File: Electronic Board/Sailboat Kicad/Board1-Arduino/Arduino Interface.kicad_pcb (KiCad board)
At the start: 2 copper layers, 70.5 x 101.6 mm, 54 parts, among them J1 Conn_01x02, J10 Conn_01x02, J11 Conn_01x03_Male, J12 Conn_01x03_Male, J13 Conn_01x03_Male, J14 Conn_01x03_Male, J15 Conn_01x04, J16 Conn_01x04, J17 Conn_01x04, J18 Conn_01x04, J19 Conn_01x03, J2 Conn_01x08, J20 Conn_01x03, J21 Conn_01x02, J22 Conn_01x02, J23 Conn_01x06, J24 Conn_01x03, J25 Conn_01x06, J26 Conn_02x02_Odd_Even, J3 Conn_01x08, J31 Conn_01x04, J32 Conn_01x04, J34 Conn_01x02, J35 Conn_01x02, J36 Conn_01x02, J37 Conn_01x02, J4 Conn_01x08, J5 Conn_02x18_Odd_Even, J6 Conn_01x08, J7 Conn_01x08, J8 Conn_01x08, J9 Conn_01x02, U1 L7805, U2 L7805, U3 L7805

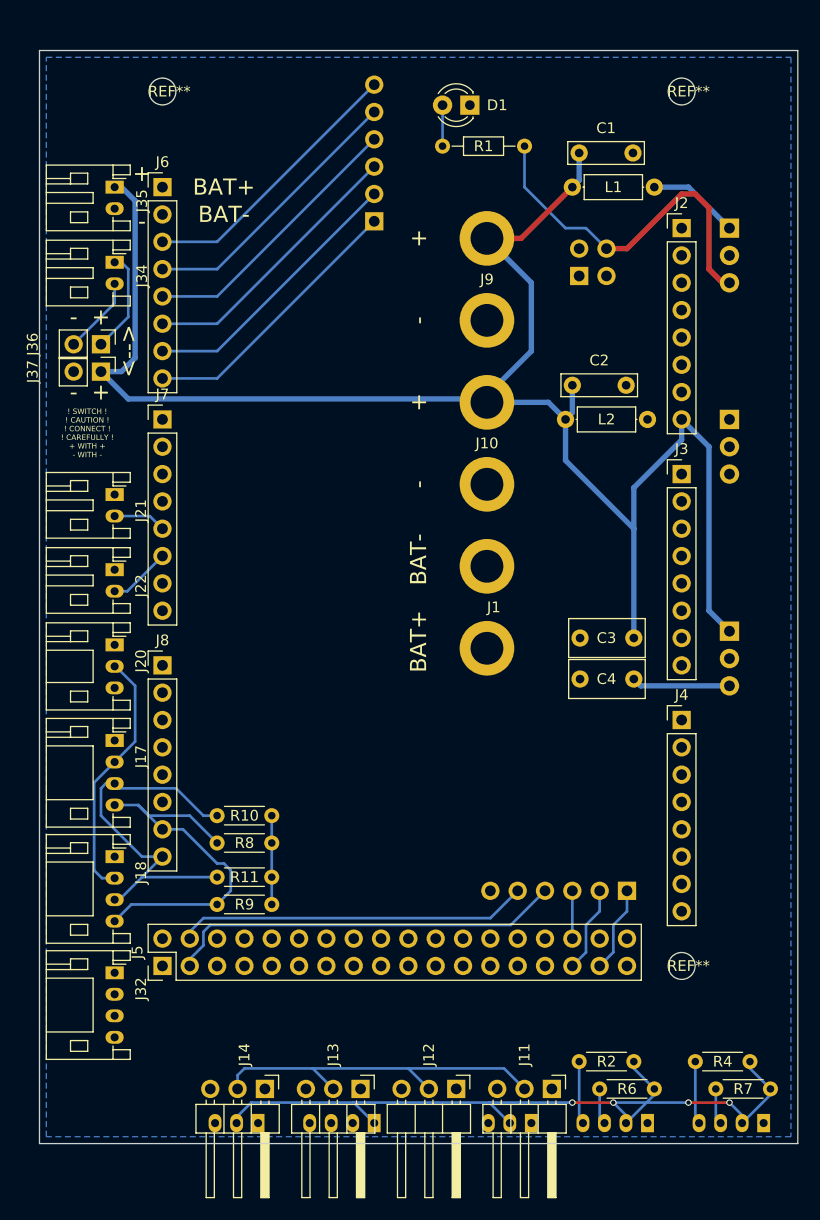
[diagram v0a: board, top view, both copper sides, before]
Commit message: Finished board-v0.1
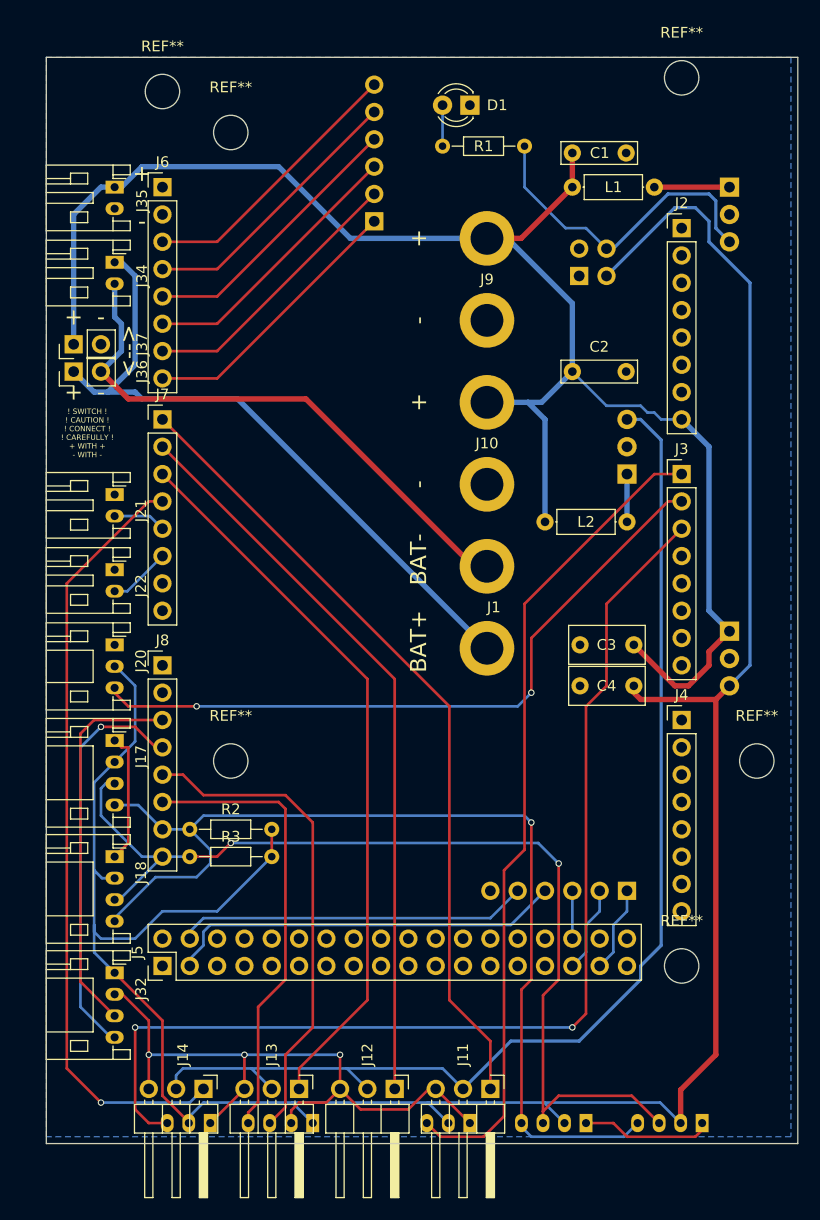
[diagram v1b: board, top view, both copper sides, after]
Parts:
- removed R10, R11, R4, R6, R7, R8, R9: 4k7, Resistors_THT:R_Axial_DIN0204_L3.6mm_D1.6mm_P5.08mm_Horizontal
- removed the REF** at (177.2, 55.9)
- removed the REF** at (128.9, 55.9)
- removed the REF** at (177.2, 137.2)
- added R3: 4k7, Resistors_THT:R_Axial_DIN0204_L3.6mm_D1.6mm_P7.62mm_Horizontal, F.Cu at (131.4, 127.0)
- added REF**: MountingHole_3.2mm_M3, Mounting_Holes:MountingHole_3.2mm_M3, F.Cu at (128.9, 55.9)
- added REF**: MountingHole_3.2mm_M3, Mounting_Holes:MountingHole_3.2mm_M3, F.Cu at (177.2, 54.6)
- added REF**: MountingHole_3.2mm_M3, Mounting_Holes:MountingHole_3.2mm_M3, F.Cu at (177.2, 137.2)
- added REF**: MountingHole_3.2mm_M3, Mounting_Holes:MountingHole_3.2mm_M3, F.Cu at (135.3, 59.7)
- added REF**: MountingHole_3.2mm_M3, Mounting_Holes:MountingHole_3.2mm_M3, F.Cu at (135.3, 118.1)
- added REF**: MountingHole_3.2mm_M3, Mounting_Holes:MountingHole_3.2mm_M3, F.Cu at (184.2, 118.1)
- R2: footprint Resistors_THT:R_Axial_DIN0204_L3.6mm_D1.6mm_P5.08mm_Horizontal -> Resistors_THT:R_Axial_DIN0204_L3.6mm_D1.6mm_P7.62mm_Horizontal
- moved R2 46.6 mm to (131.4, 124.5), turned to 0 degrees
- moved U2 10.8 mm to (172.1, 91.4), turned to 90 degrees
- moved L2 9.71 mm to (172.1, 95.9)
- moved J11 5.72 mm to (159.4, 148.6)
- moved J12 5.72 mm to (150.5, 148.6)
- moved J13 5.72 mm to (141.6, 148.6)
- moved J14 5.72 mm to (132.7, 148.6)
- moved J15 5.72 mm to (168.3, 151.8)
- moved J16 5.72 mm to (179.1, 151.8)
- moved J19 5.72 mm to (157.5, 151.8)
- moved J31 5.72 mm to (142.9, 151.8)
- moved J24 4.44 mm to (133.3, 151.8)
- moved U1 3.81 mm to (181.6, 64.8)
- moved J36 3.59 mm to (120.7, 81.9), turned to 90 degrees
- moved J37 3.59 mm to (120.7, 79.4), turned to 90 degrees
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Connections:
- R2 pad 1: /Connectors/5V-Sensors -> SDA
- R2 pad 2: SDA -> /Connectors/5V-Sensors
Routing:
- net /Connectors/5V-Sensors: track 113.4 -> 239.0 mm, vias 4 -> 0
- net A2: track 0.00 -> 102.8 mm, vias 0 -> 2
- net GND: track 0.00 -> 85.2 mm, vias 0 -> 3
- net A0: track 0.00 -> 76.5 mm
- net /Connectors/5V-Servo: track 34.4 -> 110.0 mm
- net Sail: track 0.00 -> 74.9 mm
- net Servo2: track 0.00 -> 71.7 mm, vias 0 -> 1
- net Rudder: track 0.00 -> 68.6 mm
- net Servo1: track 0.00 -> 67.7 mm
- net A1: track 0.00 -> 64.7 mm, vias 0 -> 2
- net Net-(J1-Pad1): track 9.57 -> 63.3 mm
- net SCL: track 41.9 -> 93.4 mm, vias 0 -> 2
- net SDA: track 47.7 -> 96.1 mm, vias 0 -> 1
- net TX_1: track 0.00 -> 45.6 mm
- net Net-(J1-Pad2): track 7.20 -> 52.6 mm
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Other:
- board size 70.5 x 101.6 mm -> 69.9 x 101 mm
